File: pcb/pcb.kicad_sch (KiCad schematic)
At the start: 18 parts

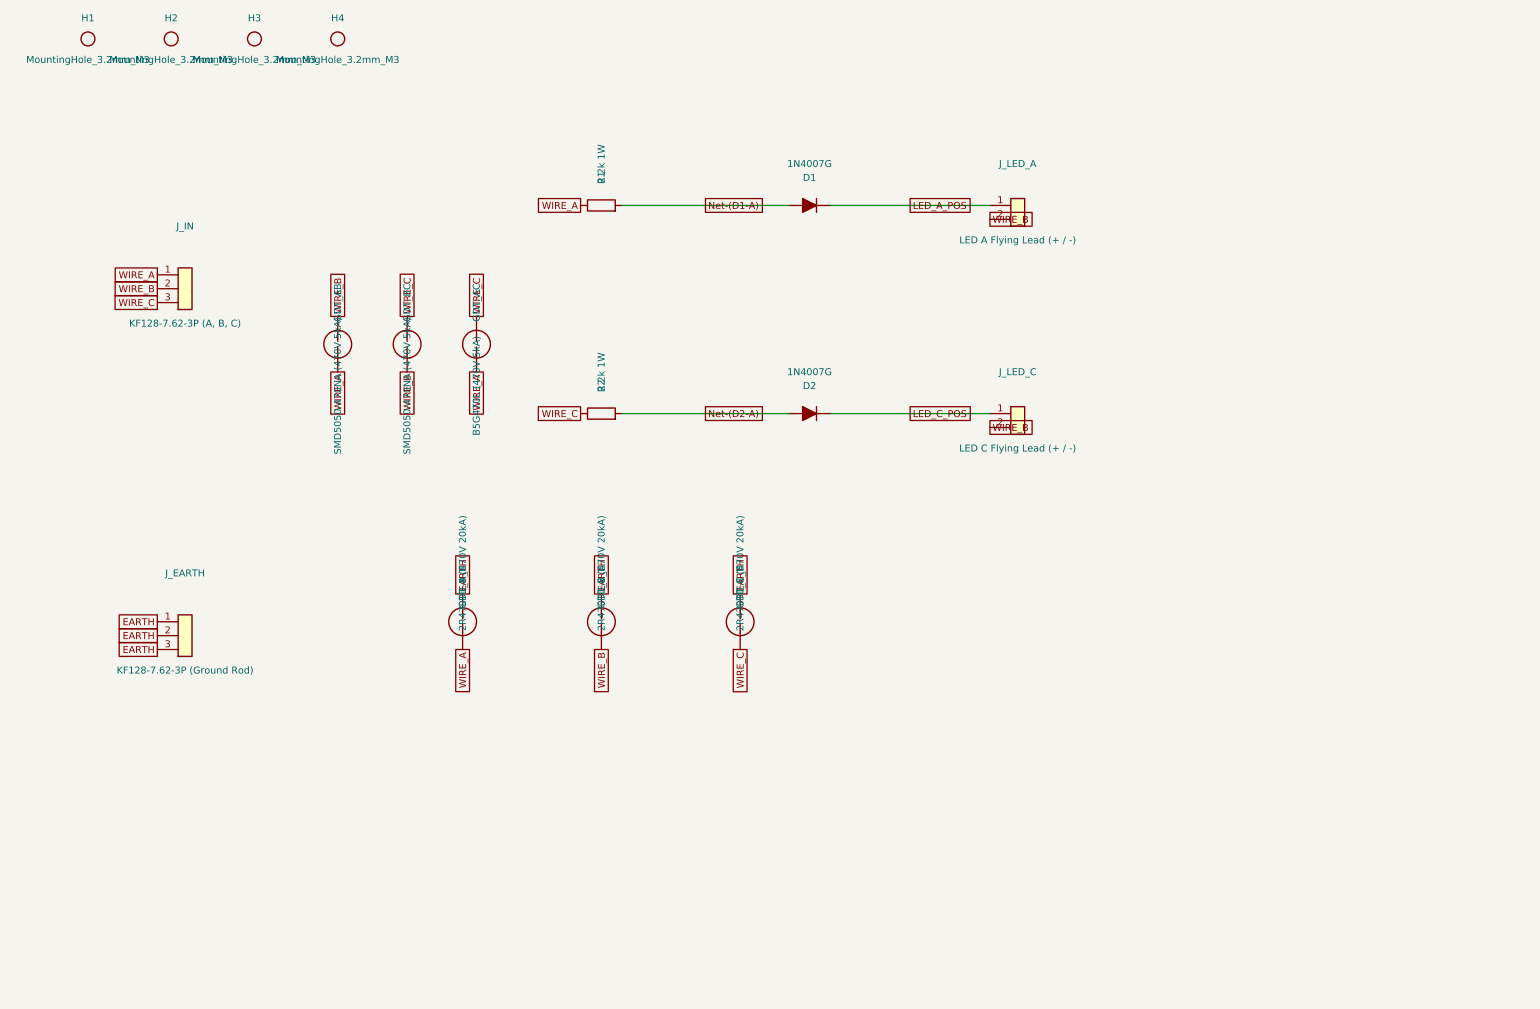
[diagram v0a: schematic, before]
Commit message: Clean up schematic for visual clarity and overlaps
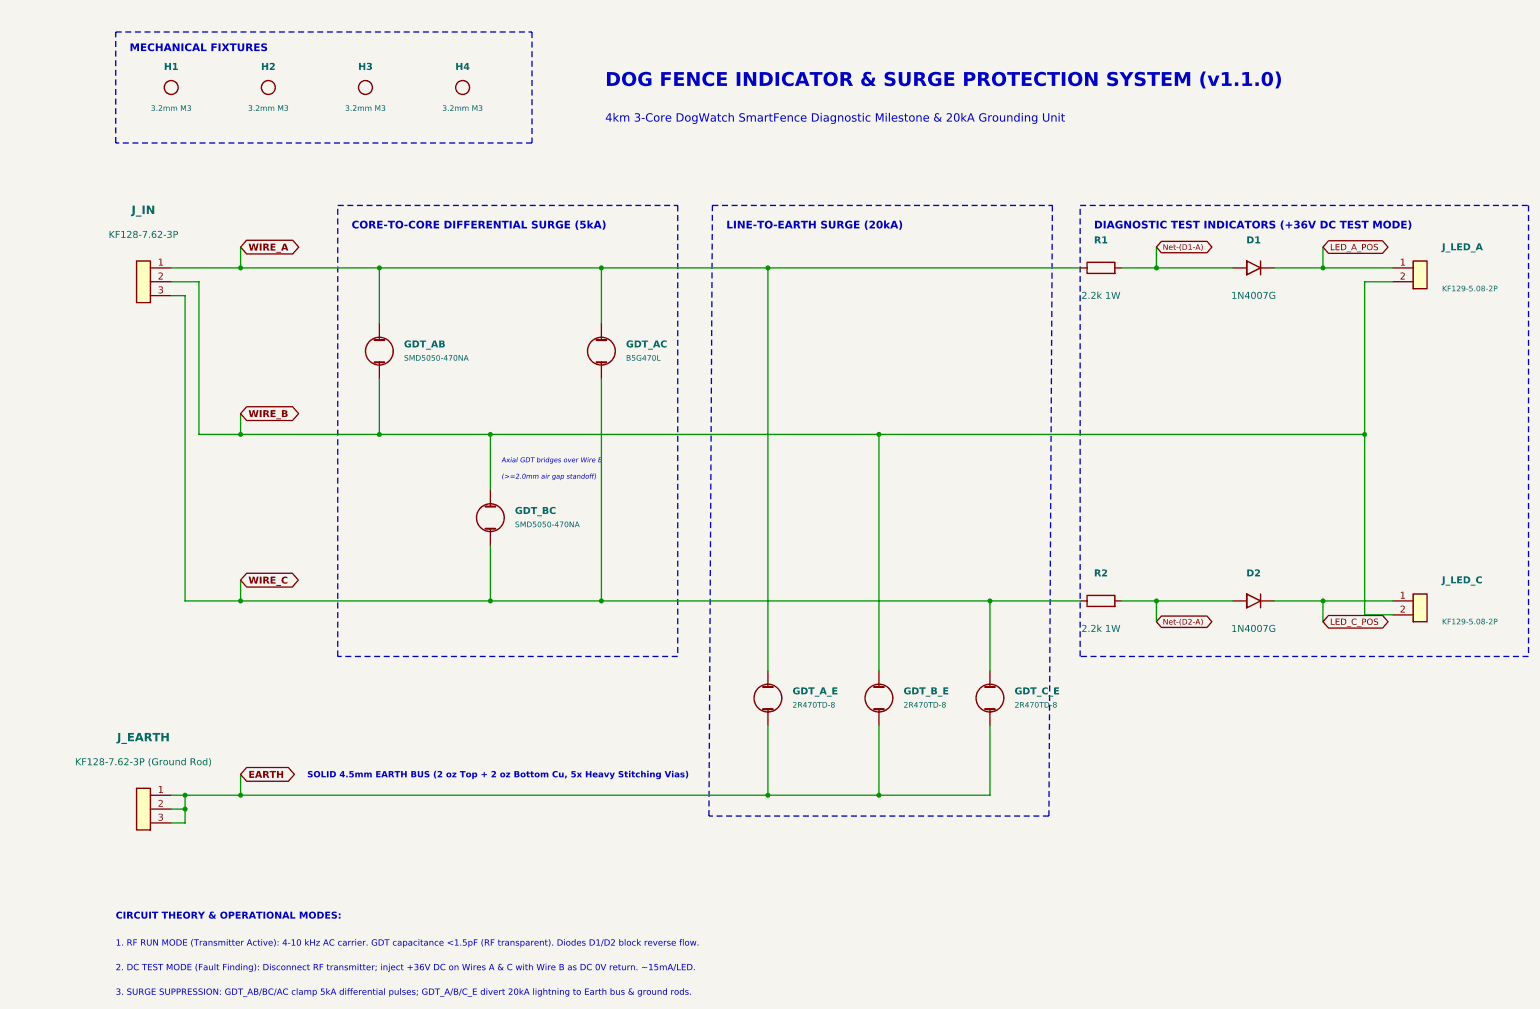
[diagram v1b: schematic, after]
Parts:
- GDT_AB, GDT_BC: value SMD5050-470NA (470V 5kA) -> SMD5050-470NA
- GDT_AC: value B5G470L (470V 5kA) -> B5G470L
- GDT_A_E, GDT_B_E, GDT_C_E: value 2R470TD-8 (470V 20kA) -> 2R470TD-8
- H1, H2, H3, H4: value MountingHole_3.2mm_M3 -> 3.2mm M3
- J_IN: value KF128-7.62-3P (A, B, C) -> KF128-7.62-3P
- J_LED_A: value LED A Flying Lead (+ / -) -> KF129-5.08-2P
- J_LED_C: value LED C Flying Lead (+ / -) -> KF129-5.08-2P
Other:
- note added: "(>=2.0mm air gap standoff)"
- note added: "1. RF RUN MODE (Transmitter Active): 4-10 kHz AC carrier. GDT capacitance <1.5pF (RF transparent). Diodes D1/D2 block reverse flow."
- note added: "2. DC TEST MODE (Fault Finding): Disconnect RF transmitter; inject +36V DC on Wires A & C with Wire B as DC 0V return. ~15mA/LED."
- note added: "3. SURGE SUPPRESSION: GDT_AB/BC/AC clamp 5kA differential pulses; GDT_A/B/C_E divert 20kA lightning to Earth bus & ground rods."
- note added: "4km 3-Core DogWatch SmartFence Diagnostic Milestone & 20kA Grounding Unit"
- note added: "Axial GDT bridges over Wire B"
- note added: "CIRCUIT THEORY & OPERATIONAL MODES:"
- note added: "CORE-TO-CORE DIFFERENTIAL SURGE (5kA)"
- note added: "DIAGNOSTIC TEST INDICATORS (+36V DC TEST MODE)"
- note added: "DOG FENCE INDICATOR & SURGE PROTECTION SYSTEM (v1.1.0)"
- note added: "LINE-TO-EARTH SURGE (20kA)"
- note added: "MECHANICAL FIXTURES"
- note added: "SOLID 4.5mm EARTH BUS (2 oz Top + 2 oz Bottom Cu, 5x Heavy Stitching Vias)"
- moved on the sheet: D1, D2, GDT_AB, GDT_AC, GDT_A_E, GDT_BC, GDT_B_E, GDT_C_E, H1, H2, H3, H4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
